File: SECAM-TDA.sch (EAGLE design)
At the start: 73 parts, among them IC1 MC34063AD

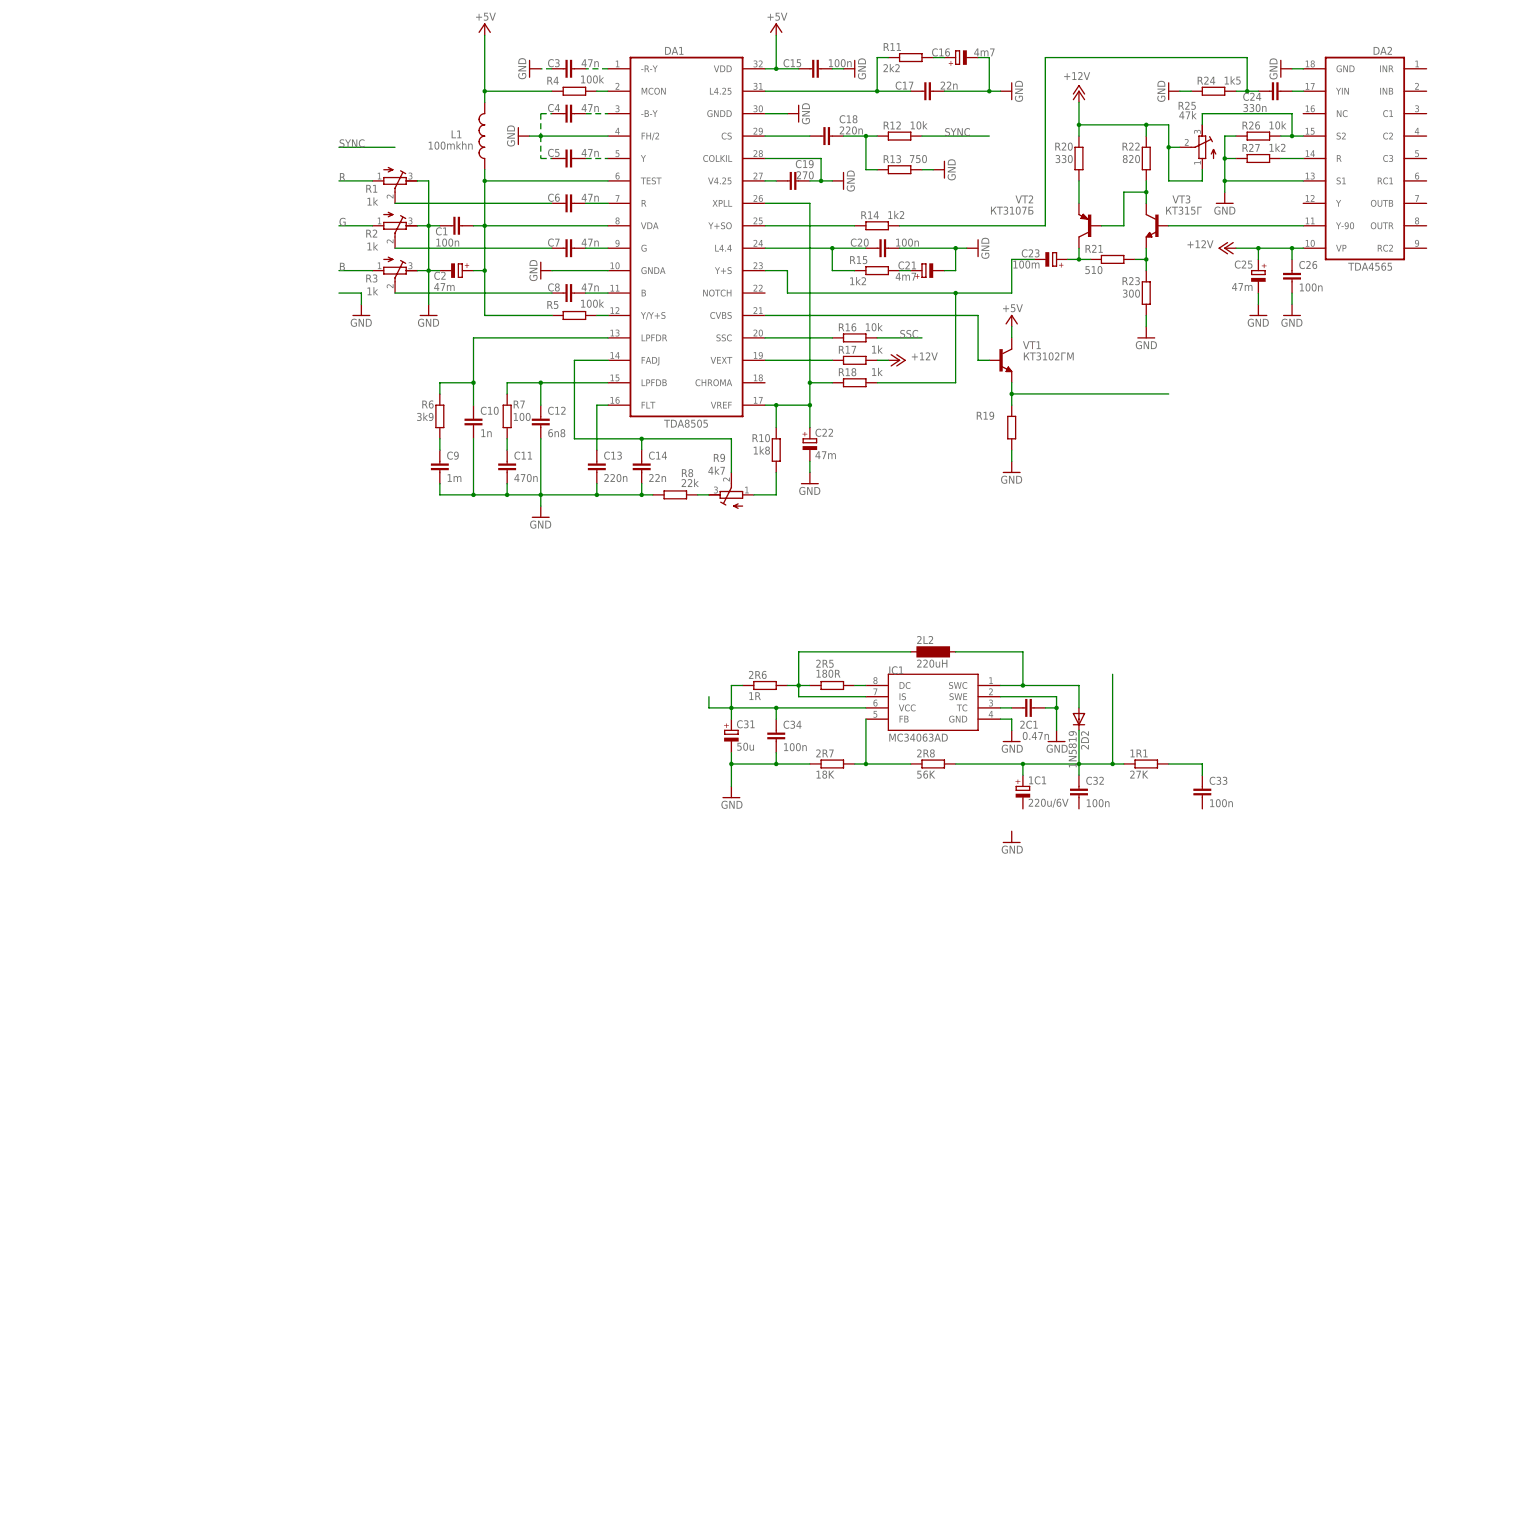
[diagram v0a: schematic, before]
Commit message: .
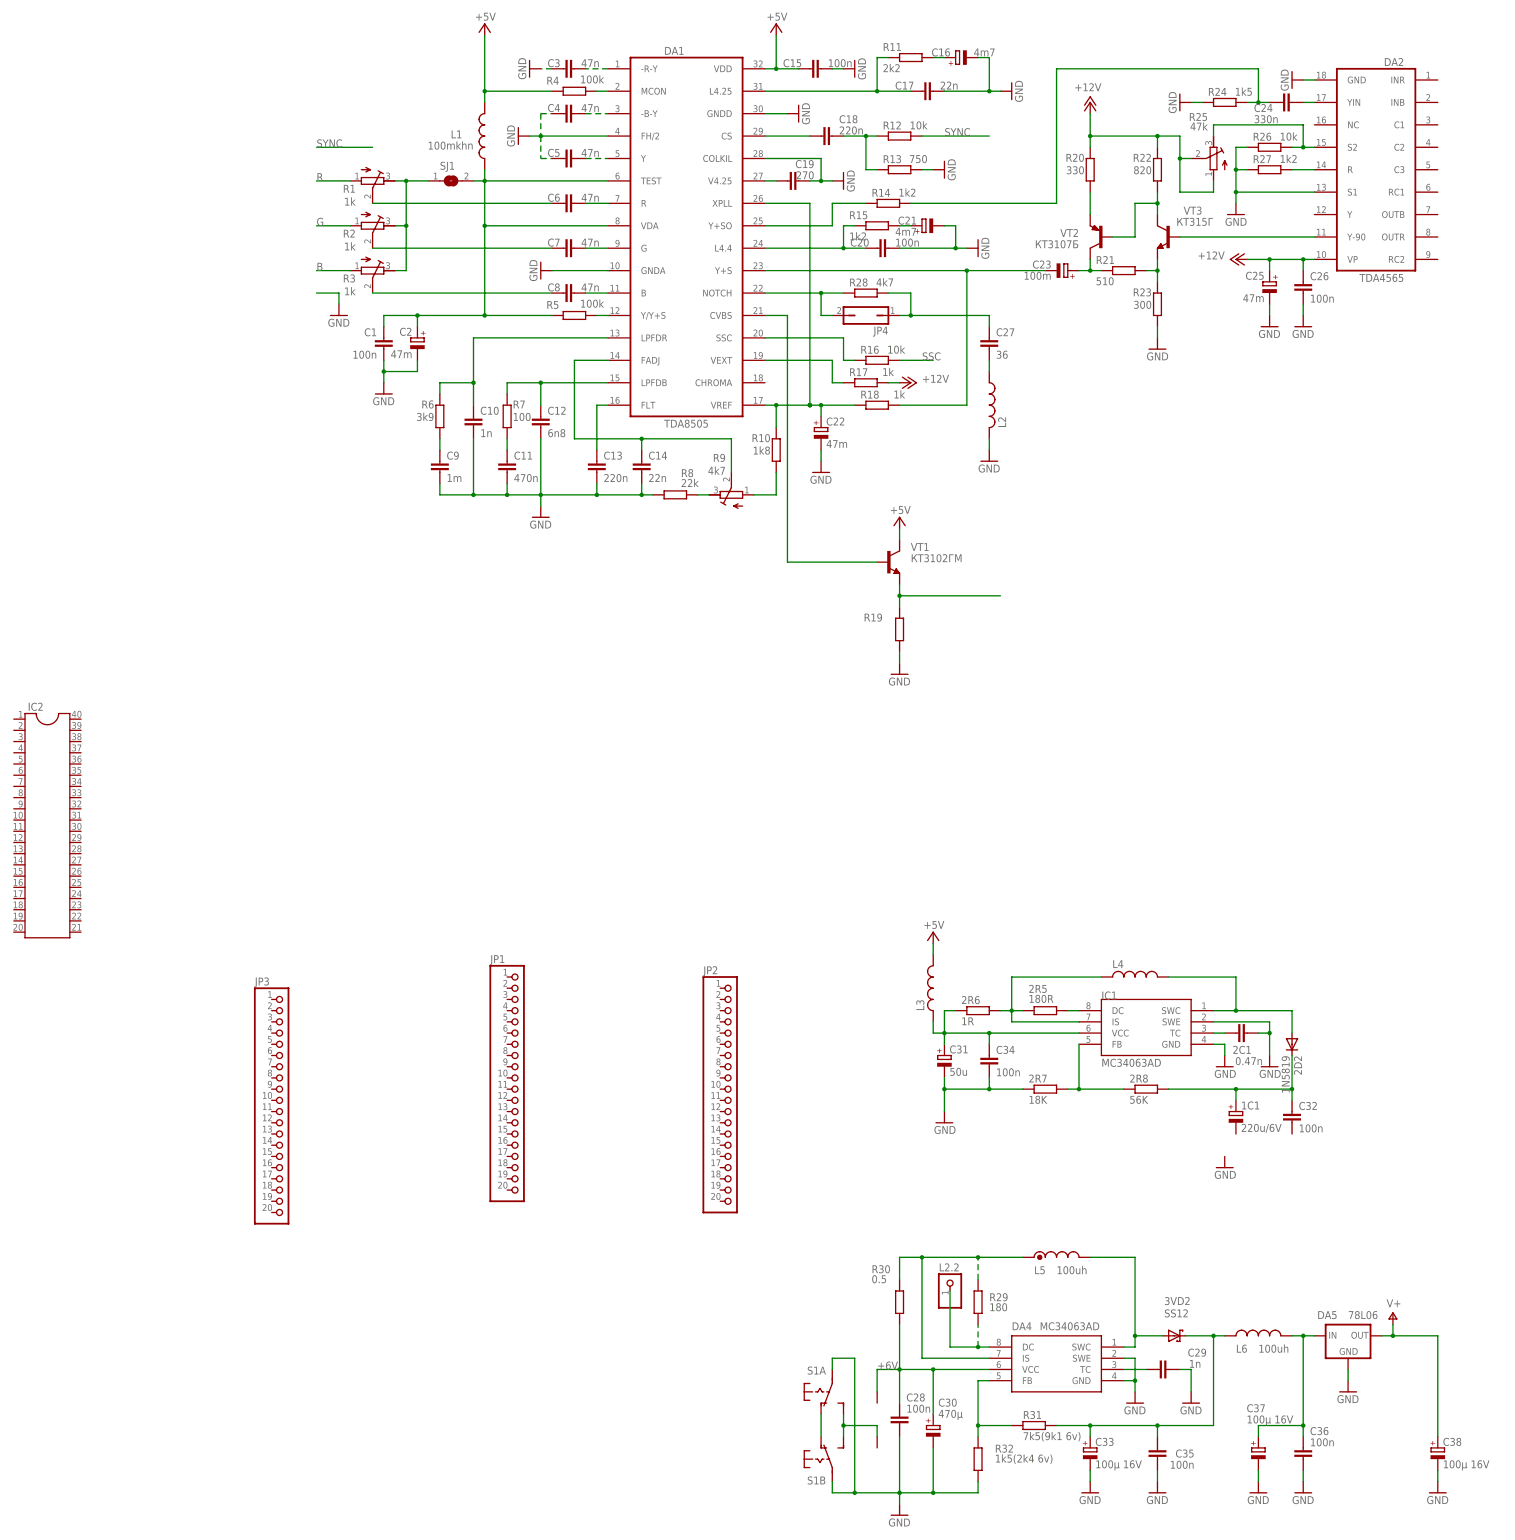
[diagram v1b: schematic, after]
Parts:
- removed 1R1: 27K, resistor:R-EU_R0805
- removed 2L2: 220uH, inductor-neosid:SD12-1000
- added 3VD2: SS12, diode:SCHOTTKY-DIODESMD
- added C27: 36, rcl:C-EUC0805
- added C28: 100n, rc-elektronik:C-EUC0805
- added C29: 1n, rcl:C-EUC0805
- added C30: 470µ, HWProgUSB:RCL_CPOL-EUE2.5-7
- added C35, C36: 100n, rcl:C-EUC0805
- added C37, C38: 100µ 16V, HWProgUSB:RCL_CPOL-EUE2.5-5
- added DA4: MC34063AD, mc34063:MC34063AD
- added DA5: 78L06, ct-pack:78LXX_SOT89
- added IC2: (no value), ic-package:DIL40
- added JP1, JP2, JP3: (no value), Разъёмы штырьковые 2.54мм:PINHD-1X20
- added JP4: (no value), jumper:JP1Q
- added L2: (no value), rcl:L0204/5
- added L2.2: (no value), pinhead:PINHD-1X1
- added L3, L4: (no value), rcl:L0204/7
- added L5: 100uh, rcl:L-US0204/7
- added L6: 100uh, rcl:L-US0207/10
- added R28: 4k7, rcl:R-EU_R0805
- added R29: 180, rcl:R-EU_M0805
- added R30: 0.5, rcl:R-EU_M1206
- added R31: 7k5(9k1 6v), rcl:R-EU_M0805
- added R32: 1k5(2k4 6v), rcl:R-EU_M0805
- added S1: SWITCH9X4, ESR_NM8032:SWITCH9X4
- added SJ1: (no value), jumper:SJ
- added U$5: B-, ESR_NM8032:B-
- added U$6: B+, ESR_NM8032:B+
- 2D2: device diode:DIODE-DO41-10 -> diode:DIODE-SMB
- C33: value 100n -> 100µ 16V; device resistor:C-EUC0805K -> HWProgUSB:RCL_CPOL-EUE2.5-5
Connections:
- new net +6V: C28.1, C30.+, DA4.VCC, R30.1, U$6.P$1
- new net N$47: C27.1, JP4.1, R28.2
- new net N$48: R1.E, R2.E, R3.E, SJ1.1
- new net N$49: DA1.NOTCH, JP4.2, R28.1
- new net N$58: C27.2, L2.2
- new net N$59: DA4.IS, L5.1, R29.2, R30.2
- new net N$60: DA4.FB, R31.1, R32.2
- new net N$61: 3VD2.A, DA4.SWC, L5.2
- new net N$62: C29.1, DA4.TC
- new net N$63: 3VD2.C, C33.+, C35.2, L6.1, R31.2
- new net N$64: S1A.S, S1B.S, U$5.P$1
- new net N$65: S1A.O, S1B.O
- new net N$66: C36.1, C37.+, DA5.IN, L6.2
- new net V+: C38.+, DA5.OUT
- net +5V: now also L3.2
- net GND: now also C1.2, C28.2, C29.2, C30.-, C33.-, C35.1, C36.2, C37.-, C38.-, DA4.GND, DA4.SWE, DA5.GND, L2.1, R32.1, S1A.P, S1B.P; no longer C1.1, R1.E, R2.E, R3.E
- net N$51: now also L4.2; no longer 2L2.2
- net N$52: now also L4.1; no longer 2L2.1
- net N$55: now also DA4.DC, L2.2.1, R29.1; no longer 1R1.2, C33.1
- net N$56: no longer 1R1.1
- net N$57: now also L3.1
- net N$6: now also C1.1, SJ1.2; no longer C1.2
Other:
- note added: "! L2.2 OR R14"
- note added: "2mm"
- note added: "4mm"
- note added: "6mm"
- note added: "8mm"
- note added: "C22 100n"
- note added: "L2 a..b 100mkhn ~47w d0.3mm b..c 11w"
- note added: "Power"
- note added: "a"
- note added: "b"
- note added: "c"
- moved on the sheet: 1C1, 2C1, 2D2, 2R5, 2R6, 2R7, 2R8, C1, C2, C21, C22, C23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
